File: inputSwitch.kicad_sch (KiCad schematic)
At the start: 5 parts

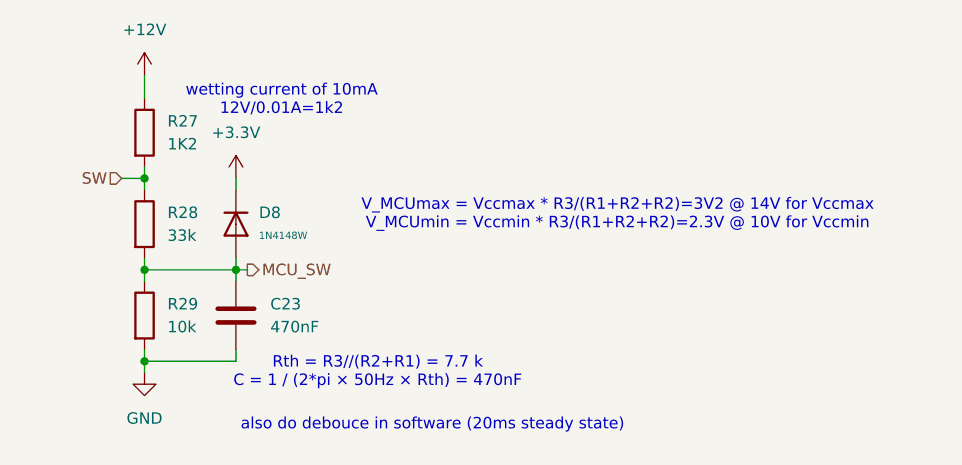
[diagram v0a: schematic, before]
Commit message: started pin assignement
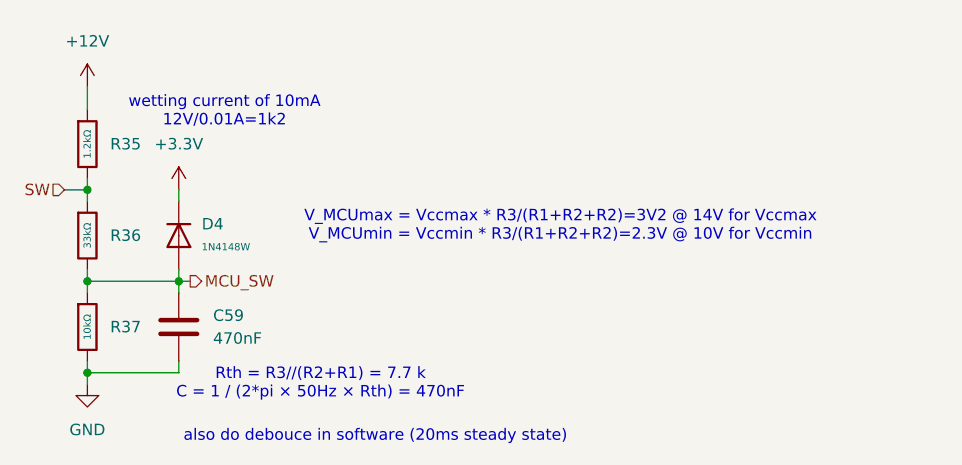
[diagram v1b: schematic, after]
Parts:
- removed C23: 470nF, symbol Device:C
- removed D8: 1N4148W, PCM_JLCPCB:D_SOD-123, symbol PCM_JLCPCB-Diodes:Switching,1N4148W
- removed R27: 1K2, symbol Device:R
- removed R28: 33k, symbol Device:R
- removed R29: 10k, symbol Device:R
- added C59: 470nF, symbol Device:C
- added D4: 1N4148W, PCM_JLCPCB:D_SOD-123, symbol PCM_JLCPCB-Diodes:Switching,1N4148W
- added R35: 1.2kΩ, PCM_JLCPCB:R_0805, symbol PCM_JLCPCB-Resistors:0805,1.2kΩ
- added R36: 33kΩ, PCM_JLCPCB:R_0805, symbol PCM_JLCPCB-Resistors:0805,33kΩ
- added R37: 10kΩ, PCM_JLCPCB:R_0805, symbol PCM_JLCPCB-Resistors:0805,10kΩ
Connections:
- net +12V: now also R35.1
- net +3.3V: now also D4.1
- net GND: now also C59.2, R37.2
- net MCU_SW: now also C59.1, D4.2, R36.2, R37.1
- net SW: now also R35.2, R36.1
